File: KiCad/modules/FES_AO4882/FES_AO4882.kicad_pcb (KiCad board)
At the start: 4 copper layers, 15 x 11 mm, 42 parts, among them J1 Conn_01x01_Pin, J10 Conn_01x01_Pin, J11 Conn_01x01_Pin, J12 Conn_01x01_Pin, J13 Conn_01x01_Pin, J14 Conn_01x01_Pin, J15 Conn_01x01_Pin, J16 Conn_01x01_Pin, J17 Conn_01x01_Pin, J18 Conn_01x01_Pin, J19 Conn_01x01_Pin, J2 Conn_01x01_Pin, J20 Conn_01x01_Pin, J21 Conn_01x01_Pin, J22 Conn_01x01_Pin, J23 Conn_01x01_Pin, J24 Conn_01x01_Pin, J3 Conn_01x01_Pin, J4 Conn_01x01_Pin, J5 Conn_01x01_Pin, J6 Conn_01x01_Pin, J7 Conn_01x01_Pin, J8 Conn_01x01_Pin, J9 Conn_01x01_Pin, Q1 AO4882_C3040598, Q2 AO4882_C3040598, SW1 TS-1088R-02026, U1 DS12W-MS, U2 DS12W-MS, U3 DS12W-MS, U4 HC32L110C6UA-SFN20TR, U5 DS12W-MS

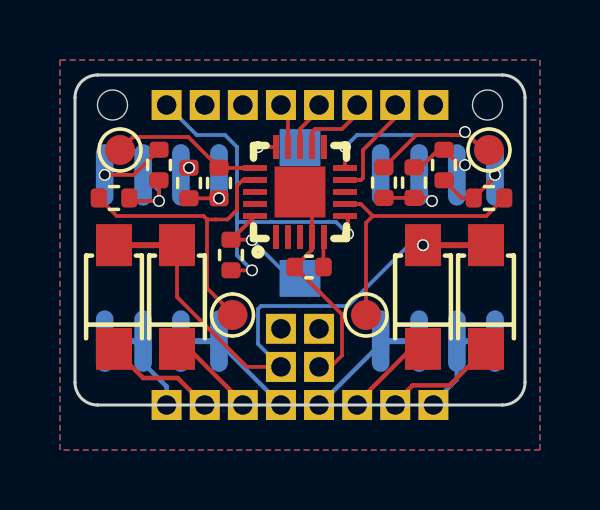
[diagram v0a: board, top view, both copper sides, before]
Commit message: cleaned all modules + production files
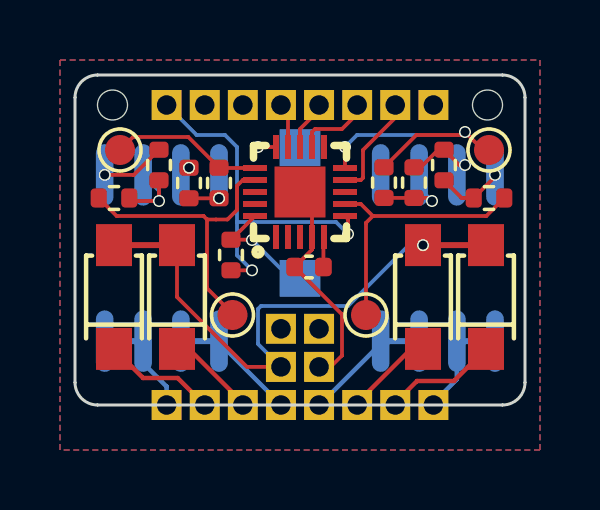
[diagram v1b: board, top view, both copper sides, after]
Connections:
- net /SWCLK/IO1out renamed /SWCLK
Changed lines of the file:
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@@
 	(net 8 "/SCLK_ARM")
 	(net 9 "/SPICS_ARM")
-	(net 10 "/SWCLK{slash}IO1out")
+	(net 10 "/SWCLK")
 	(net 11 "/GPIO")
 	(net 12 "VCC")
@@
 		(sheetname "Root")
 		(sheetfile "FES_AO4882.kicad_sch")
-		(attr through_hole)
+		(attr through_hole exclude_from_bom dnp)
 		(fp_line
 			(start -1.05 -0.11)
@@
 			(size 1 1)
 			(drill 0.65)
+			(property pad_prop_castellated)
 			(layers "*.Cu" "*.Mask")
 			(remove_unused_layers no)
@@
 			(size 0.2 0.8)
 			(layers "F.Cu" "F.Paste" "F.Mask")
-			(net 10 "/SWCLK{slash}IO1out")
+			(net 10 "/SWCLK")
 			(pinfunction "SWCLK")
 			(pintype "input")
@@
 		(sheetname "Root")
 		(sheetfile "FES_AO4882.kicad_sch")
-		(attr through_hole)
+		(attr through_hole exclude_from_bom dnp)
 		(fp_line
 			(start -1.05 -0.11)
@@
 			(size 1 1)
 			(drill 0.65)
+			(property pad_prop_castellated)
 			(layers "*.Cu" "*.Mask")
 			(remove_unused_layers no)
@@
 		(sheetname "Root")
 		(sheetfile "FES_AO4882.kicad_sch")
-		(attr through_hole)
+		(attr through_hole exclude_from_bom dnp)
 		(fp_line
 			(start -1.05 -0.11)
@@
 			(size 1 1)
 			(drill 0.65)
+			(property pad_prop_castellated)
 			(layers "*.Cu" "*.Mask")
 			(remove_unused_layers no)
@@
 		(sheetname "Root")
 		(sheetfile "FES_AO4882.kicad_sch")
-		(attr through_hole)
+		(attr through_hole exclude_from_pos_files exclude_from_bom dnp)
 		(fp_line
 			(start -1.05 -0.11)
@@
 			(size 1 1)
 			(drill 0.65)
+			(property pad_prop_castellated)
 			(layers "*.Cu" "*.Mask")
 			(remove_unused_layers no)
@@
 		(sheetname "Root")
 		(sheetfile "FES_AO4882.kicad_sch")
-		(attr through_hole)
+		(attr through_hole exclude_from_bom dnp)
 		(fp_line
 			(start -1.05 -0.11)
@@
 			(size 1 1)
 			(drill 0.65)
+			(property pad_prop_castellated)
 			(layers "*.Cu" "*.Mask")
 			(remove_unused_layers no)
@@
 		(sheetname "Root")
 		(sheetfile "FES_AO4882.kicad_sch")
-		(attr through_hole)
+		(attr through_hole exclude_from_bom dnp)
 		(fp_line
 			(start -1.05 -0.11)
@@
 			(size 1 1)
 			(drill 0.65)
+			(property pad_prop_castellated)
 			(layers "*.Cu" "*.Mask")
 			(remove_unused_layers no)
@@
 			(layers "*.Cu" "*.Mask")
 			(remove_unused_layers no)
-			(net 10 "/SWCLK{slash}IO1out")
+			(net 10 "/SWCLK")
 			(pinfunction "Pin_1")
 			(pintype "passive")
@@
 		(sheetname "Root")
 		(sheetfile "FES_AO4882.kicad_sch")
-		(attr through_hole)
+		(attr through_hole exclude_from_bom dnp)
 		(fp_line
 			(start -1.05 -0.11)
@@
 			(size 1 1)
 			(drill 0.65)
+			(property pad_prop_castellated)
 			(layers "*.Cu" "*.Mask")
 			(remove_unused_layers no)
@@
 		(sheetname "Root")
 		(sheetfile "FES_AO4882.kicad_sch")
-		(attr through_hole)
+		(attr through_hole exclude_from_bom dnp)
 		(fp_line
 			(start -1.05 -0.11)
@@
 			(size 1 1)
 			(drill 0.65)
+			(property pad_prop_castellated)
 			(layers "*.Cu" "*.Mask")
 			(remove_unused_layers no)
@@
 	)
 	(segment
-		(start 34.9835 34.3465)
-		(end 33.754999 34.3465)
+		(start 36.2 33.13)
+		(end 35.13 34.2)
 		(width 0.15)
 		(layer "F.Cu")
@@
 	)
 	(segment
-		(start 33.754999 34.3465)
+		(start 33.901499 34.2)
 		(end 33.175 34.926499)
 		(width 0.15)
@@
 	)
 	(segment
-		(start 36.2 33.13)
-		(end 34.9835 34.3465)
+		(start 35.13 34.2)
+		(end 33.901499 34.2)
 		(width 0.15)
 		(layer "F.Cu")
